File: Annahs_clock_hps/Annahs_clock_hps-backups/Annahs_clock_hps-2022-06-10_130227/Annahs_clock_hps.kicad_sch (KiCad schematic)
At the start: 19 parts, among them J1 PJ-102AH, Y1 Crystal 22p

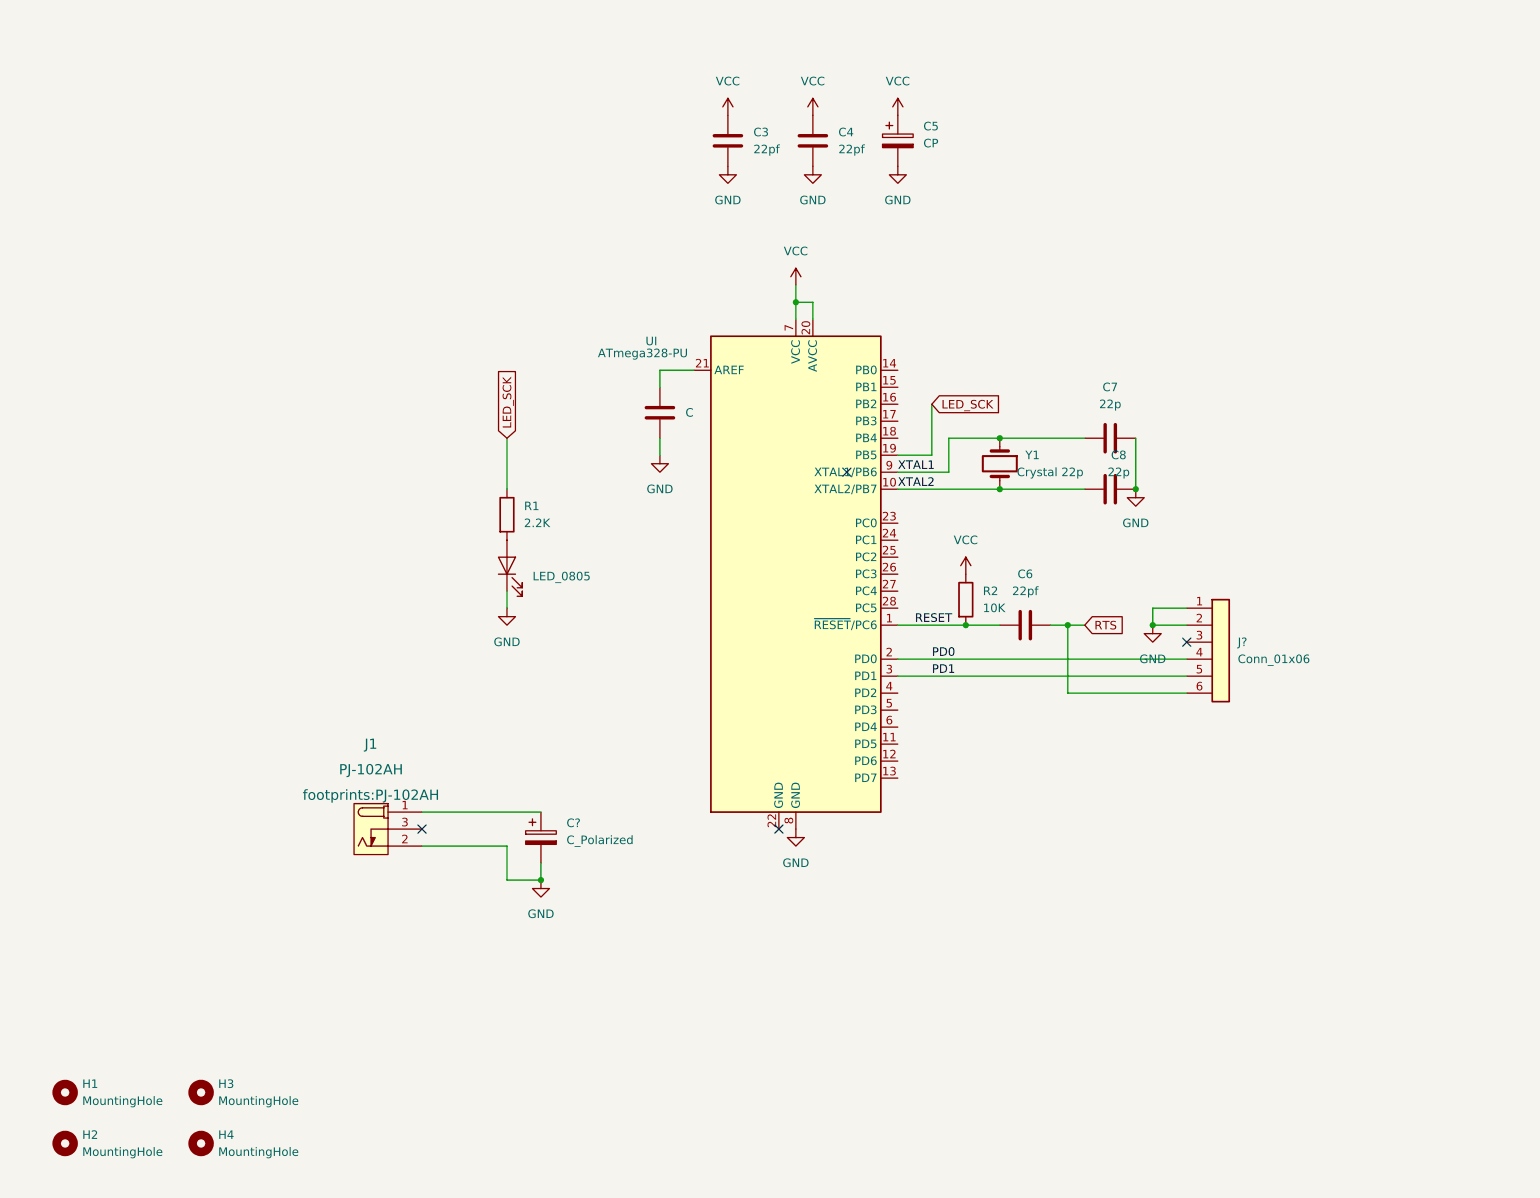
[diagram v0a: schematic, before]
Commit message: Week 1/2 Schematic Update
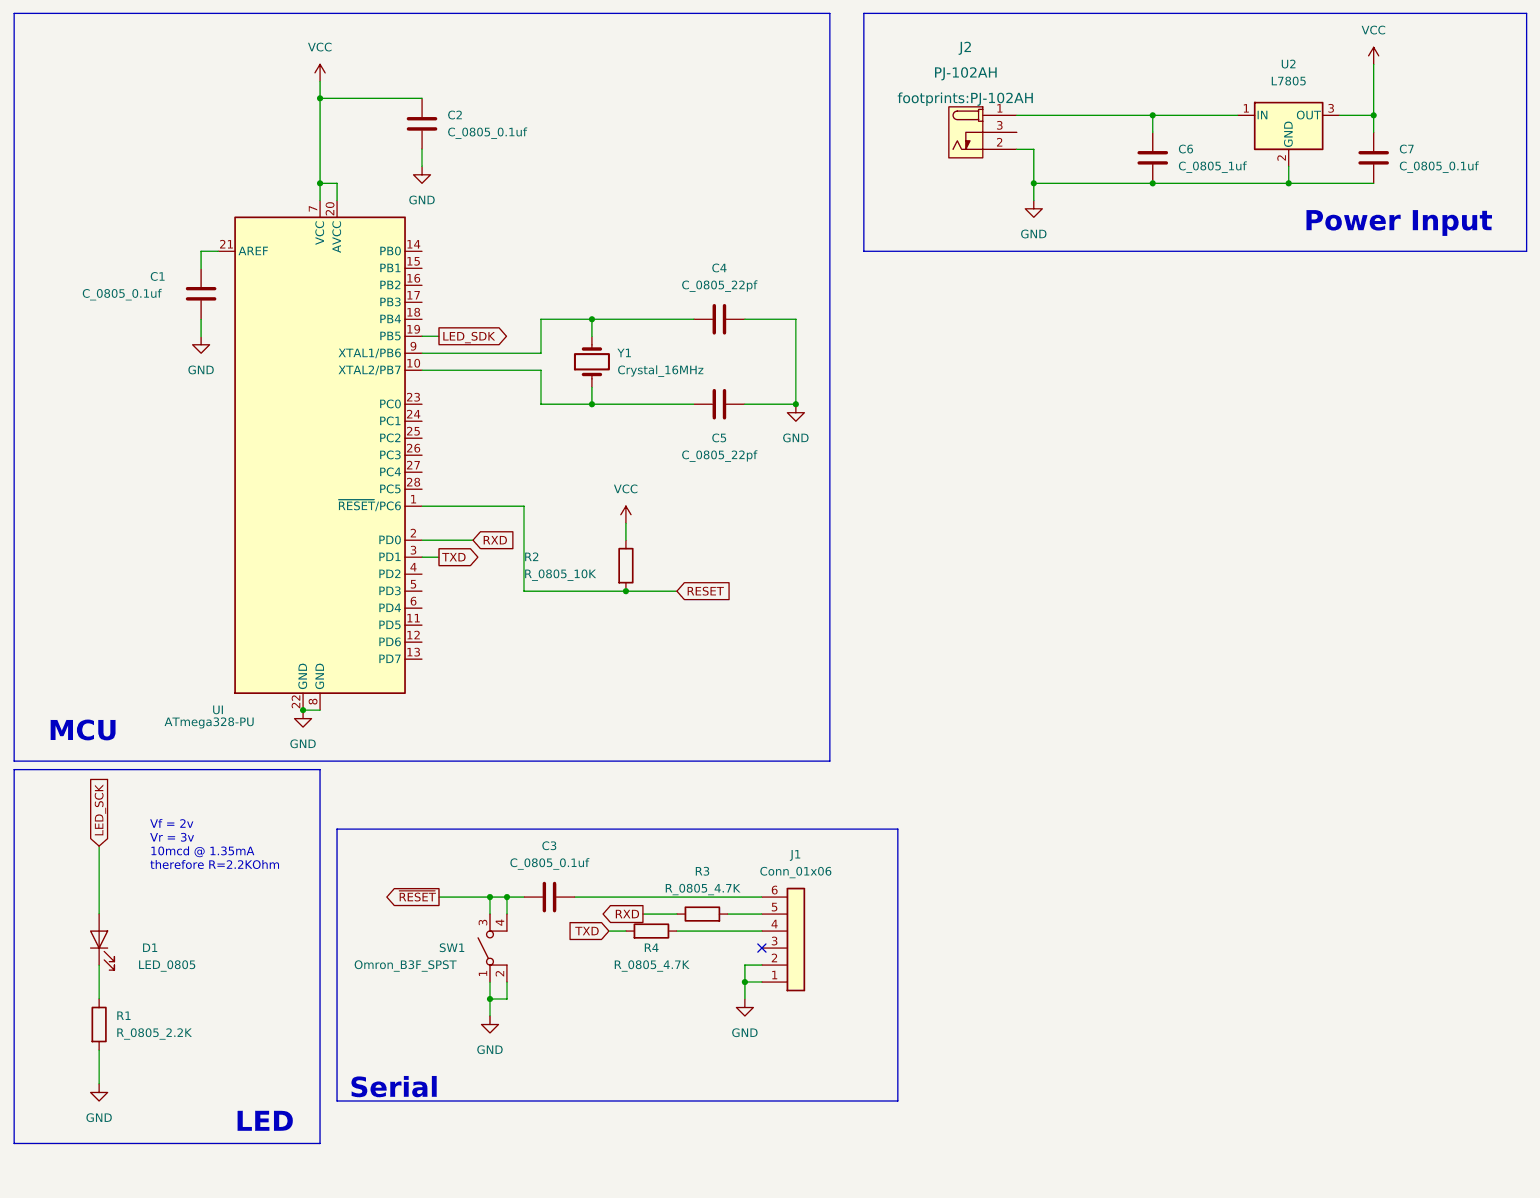
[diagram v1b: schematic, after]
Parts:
- removed C: C_0805_22pf, footprints:C_0805_2012Metric, symbol HPS:C_0805_22pf
- removed C3, C6: 22pf, footprints:C_0805_2012Metric, symbol HPS:C_0805_22pf
- removed C5: CP, symbol KICAD:C_Polarized
- removed C7, C8: 22p, footprints:C_0805_2012Metric, symbol HPS:C_0805_22pf
- removed C?: C_Polarized, symbol KICAD:C_Polarized
- removed D?: LED_0805, footprints:LED_0805_2012Metric, symbol HPS:LED_0805
- removed H1, H2, H3, H4: MountingHole, footprints:MountingHole_3.2mm_M3, symbol HPS:MountingHole
- removed J1: PJ-102AH, footprints:PJ-102AH, symbol HPS:PJ-102AH
- removed J?: Conn_01x06, footprints:PinHeader_1x06_P2.54mm_Vertical, symbol HPS:Conn_01x06
- added C1, C2, C3, C7: C_0805_0.1uf, footprints:C_0805_2012Metric, symbol HPS:C_0805_0.1uf
- added C5: C_0805_22pf, footprints:C_0805_2012Metric, symbol HPS:C_0805_22pf
- added C6: C_0805_1uf, footprints:C_0805_2012Metric, symbol HPS:C_0805_1uf
- added D1: LED_0805, footprints:LED_0805_2012Metric, symbol HPS:LED_0805
- added J1: Conn_01x06, footprints:PinHeader_1x06_P2.54mm_Vertical, symbol HPS:Conn_01x06
- added J2: PJ-102AH, footprints:PJ-102AH, symbol HPS:PJ-102AH
- added R3, R4: R_0805_4.7K, footprints:R_0805_2012Metric, symbol HPS:R_0805_4.7K
- added SW1: Omron_B3F_SPST, footprints:SW_SPST_Omron_B3FS-100xP, symbol HPS:Omron_B3F_SPST
- added U2: L7805, symbol HPS_2:L7805
- C4: value 22pf -> C_0805_22pf
- R1: value 2.2K -> R_0805_2.2K
- R2: value 10K -> R_0805_10K
- Y1: value Crystal 22p -> Crystal_16MHz
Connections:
- net GND: now also C4.1, R1.2, UI.22 (GND), C1.2, C2.2, C5.2, C6.2, C7.2, J1.1 (Pin_1), J1.2 (Pin_2), J2.2 (OUT), SW1.1 (A), SW1.2 (A), U2.2 (GND); no longer C4.2
- net LED_SCK: now also D1.2 (A); no longer R1.1, UI.19 (PB5)
- net VCC: now also C2.1, C7.1, U2.3 (OUT); no longer C4.1
- net at UI.21 (AREF): now also C1.1
- net PD0 renamed RXD
- net RXD: now also R3.1
- net PD1 renamed TXD
- net TXD: now also R4.2
- net XTAL1: no longer names the net of Y1.1
- net XTAL1: now also UI.10 (XTAL2/PB7), C5.1; no longer UI.9 (XTAL1/PB6)
- net XTAL2: no longer names the net of Y1.2
- net XTAL2: now also C4.2, UI.9 (XTAL1/PB6); no longer UI.10 (XTAL2/PB7)
- new net: D1.1 (K), R1.1
- new net: J1.5 (Pin_5), R3.2
- new net: C6.1, J2.1 (POLE), U2.1 (IN)
- new net: J1.4 (Pin_4), R4.1
- new net: C3.2, J1.6 (Pin_6)
- new net LED_SDK: UI.19 (PB5)
- new net ~{RESET}: C3.1, SW1.3 (B), SW1.4 (B)
- no-connect marks 4 -> 1
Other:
- note added: "LED"
- note added: "MCU"
- note added: "Power Input"
- note added: "Serial"
- note added: "Vf = 2v Vr = 3v 10mcd @ 1.35mA therefore R=2.2KOhm"
- moved on the sheet: UI

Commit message: Clock Schematic
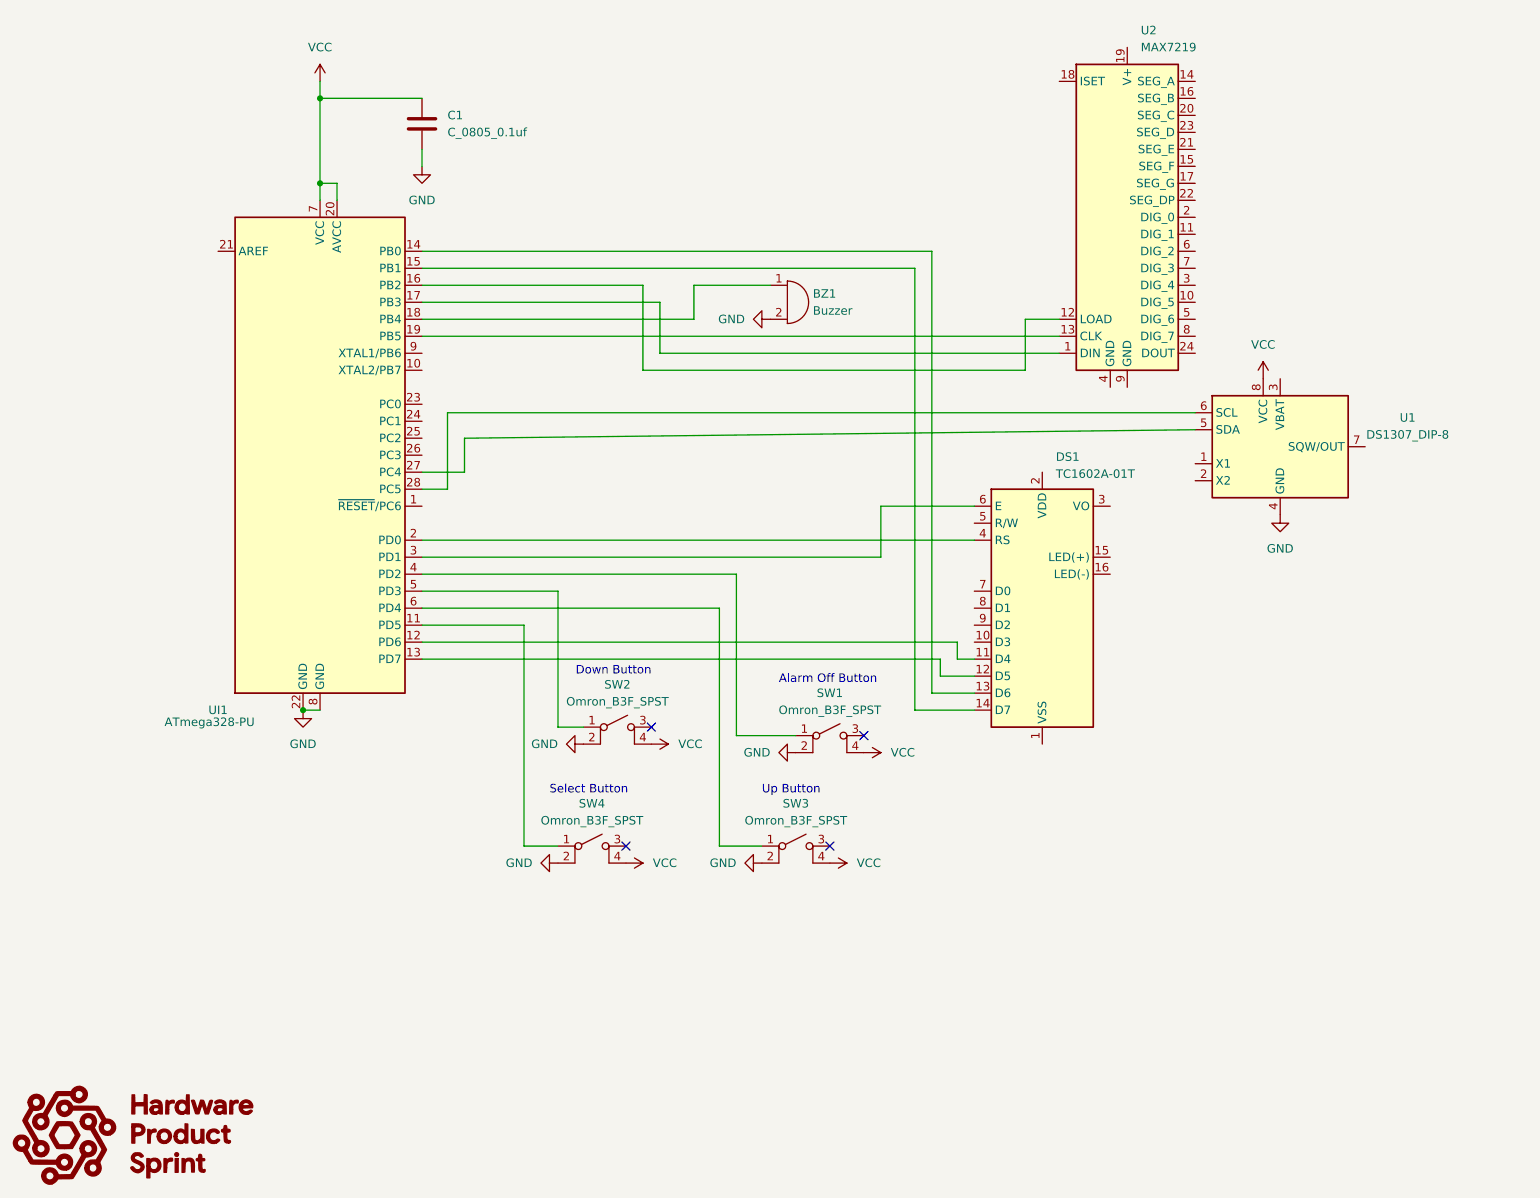
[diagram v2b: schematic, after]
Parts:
- removed C1, C3, C7: C_0805_0.1uf, footprints:C_0805_2012Metric, symbol HPS:C_0805_0.1uf
- removed C4, C5: C_0805_22pf, footprints:C_0805_2012Metric, symbol HPS:C_0805_22pf
- removed C6: C_0805_1uf, footprints:C_0805_2012Metric, symbol HPS:C_0805_1uf
- removed D1: LED_0805, footprints:LED_0805_2012Metric, symbol HPS:LED_0805
- removed J1: Conn_01x06, footprints:PinHeader_1x06_P2.54mm_Vertical, symbol HPS:Conn_01x06
- removed J2: PJ-102AH, footprints:PJ-102AH, symbol HPS:PJ-102AH
- removed R1: R_0805_2.2K, footprints:R_0805_2012Metric, symbol HPS:R_0805_2.2K
- removed R2: R_0805_10K, footprints:R_0805_2012Metric, symbol HPS:R_0805_10K
- removed R3, R4: R_0805_4.7K, footprints:R_0805_2012Metric, symbol HPS:R_0805_4.7K
- removed SW1: Omron_B3F_SPST, footprints:SW_SPST_Omron_B3FS-100xP, symbol HPS:Omron_B3F_SPST
- removed U2: L7805, symbol HPS_2:L7805
- removed Y1: Crystal_16MHz, footprints:Crystal_SMD_HC49-SD, symbol HPS:Crystal_16MHz
- added BZ1: Buzzer, footprints:Buzzer_TDK_PS1240P02BT_D12.2mm_H6.5mm, symbol HPS:Buzzer
- added DS1: TC1602A-01T, footprints:TC1602A-01T, symbol HPS:TC1602A-01T
- added SW1, SW2, SW3, SW4: Omron_B3F_SPST, footprints:SW_SPST_Omron_B3FS-100xP, symbol HPS_3:Omron_B3F_SPST
- added U1: DS1307_DIP-8, footprints:DIP-8_W7.62mm, symbol HPS:DS1307_DIP-8
- added U2: MAX7219, footprints:DIP-24_W7.62mm, symbol HPS:MAX7219
- renumbered C2 to C1, UI to UI1
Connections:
- net GND: now also BZ1.2 (+), SW1.2 (A), SW2.2 (A), SW3.2 (A), SW4.2 (A), U1.4 (GND)
- net VCC: now also SW1.4 (B), SW2.4 (B), SW3.4 (B), SW4.4 (B), U1.8 (VCC)
- net at UI1.11 (PD5): now also SW4.1 (A)
- net at UI1.12 (PD6): now also DS1.11 (D4)
- net at UI1.13 (PD7): now also DS1.12 (D5)
- net at UI1.14 (PB0): now also DS1.13 (D6)
- net at UI1.15 (PB1): now also DS1.14 (D7)
- net at UI1.16 (PB2): now also U2.12 (LOAD)
- net at UI1.17 (PB3): now also U2.1 (DIN)
- net at UI1.18 (PB4): now also BZ1.1 (-)
- net at UI1.27 (PC4): now also U1.5 (SDA)
- net at UI1.28 (PC5): now also U1.6 (SCL)
- net at UI1.4 (PD2): now also SW1.1 (A)
- net at UI1.5 (PD3): now also SW2.1 (A)
- net at UI1.6 (PD4): now also SW3.1 (A)
- net LED_SDK: no longer names the net of UI1.19 (PB5)
- net LED_SDK: now also U2.13 (CLK)
- net RESET: no longer names the net of UI1.1 (~{RESET}/PC6)
- net RXD: no longer names the net of UI1.2 (PD0)
- net RXD: now also DS1.4 (RS)
- net TXD: no longer names the net of UI1.3 (PD1)
- net TXD: now also DS1.6 (E)
- no-connect marks 1 -> 4
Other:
- note added: "Alarm Off Button"
- note added: "Down Button"
- note added: "Select Button"
- note added: "Up Button"
- note removed: "LED"
- note removed: "MCU"
- note removed: "Power Input"
- note removed: "Serial"
- note removed: "Vf = 2v Vr = 3v 10mcd @ 1.35mA therefore R=2.2KOhm"
